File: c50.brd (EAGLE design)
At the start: 95.6 x 31.1 mm, 15 parts, among them IC1 7805TV, IC2 UA555N

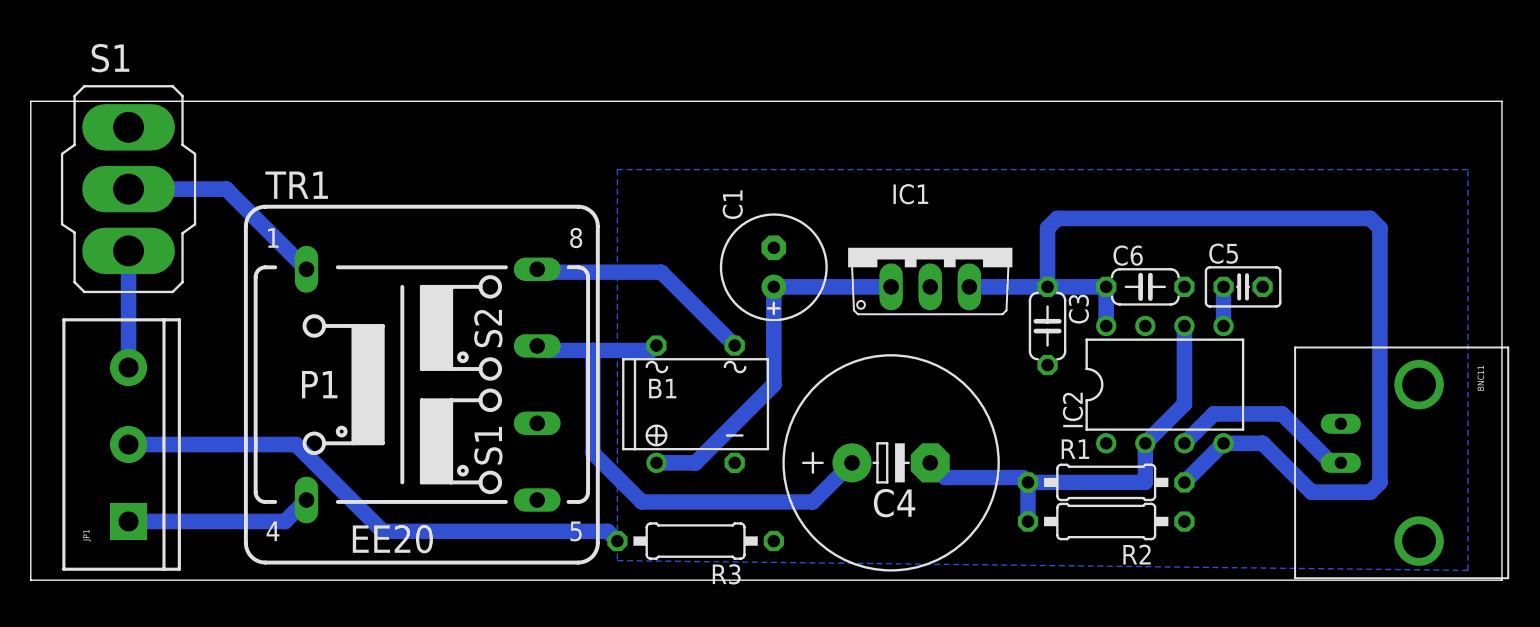
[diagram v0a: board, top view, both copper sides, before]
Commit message: Signature added.
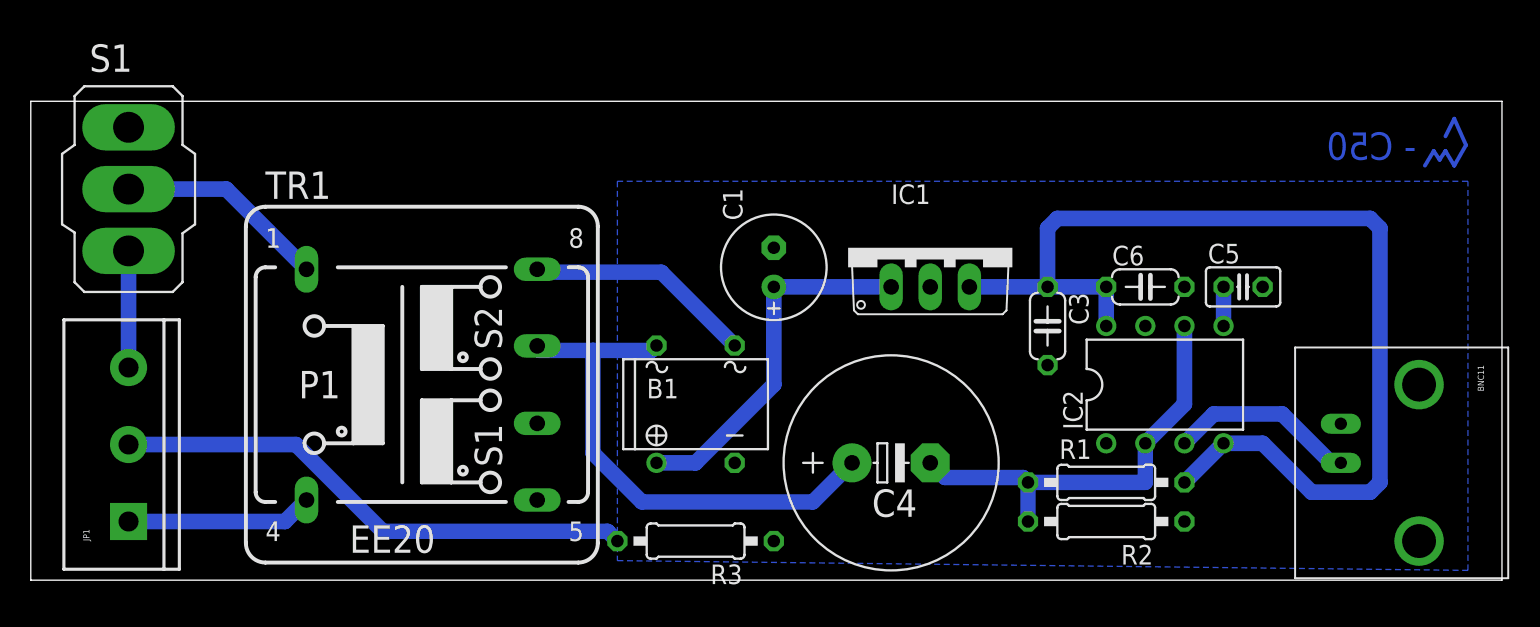
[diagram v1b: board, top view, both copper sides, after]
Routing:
- net N$11: track 0.00 -> 8.29 mm
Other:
- board text added: "- C50"
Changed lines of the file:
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@@
 <setting verticaltext="up"/>
 </settings>
-<grid distance="0.05" unitdist="inch" unit="inch" style="lines" multiple="1" display="yes" altdistance="0.0125" altunitdist="inch" altunit="inch"/>
+<grid distance="0.005" unitdist="inch" unit="inch" style="lines" multiple="1" display="yes" altdistance="0.0125" altunitdist="inch" altunit="inch"/>
 <layers>
 <layer number="1" name="Top" color="4" fill="1" visible="yes" active="yes"/>
@@
 <dimension x1="0" y1="0" x2="0" y2="31.105" x3="-4.445" y3="15.5525" textsize="1.778" layer="20"/>
 <dimension x1="0" y1="0" x2="95.555" y2="0" x3="47.7775" y3="-5.08" textsize="1.778" layer="20"/>
+<text x="90.678" y="27.305" size="1.778" layer="16" rot="MR0"> - C50</text>
 </plain>
 <attributes>
@@
 <contactref element="R3" pad="1"/>
 <polygon width="0.4064" layer="16">
-<vertex x="38.1" y="26.67"/>
+<vertex x="38.1" y="25.908"/>
 <vertex x="38.1" y="1.27"/>
 <vertex x="93.345" y="0.635"/>
-<vertex x="93.345" y="26.67"/>
+<vertex x="93.345" y="25.908"/>
 </polygon>
 </signal>
@@
 <wire x1="6.35" y1="13.81" x2="6.35" y2="21.3868" width="1.016" layer="16"/>
 </signal>
+<signal name="N$11">
+<wire x1="91.8845" y1="28.829" x2="92.456" y2="29.972" width="0.254" layer="16"/>
+<wire x1="92.456" y1="29.972" x2="93.218" y2="28.2575" width="0.254" layer="16"/>
+<wire x1="93.218" y1="28.2575" x2="92.456" y2="26.924" width="0.254" layer="16"/>
+<wire x1="92.456" y1="26.924" x2="91.8845" y2="27.8765" width="0.254" layer="16"/>
+<wire x1="91.8845" y1="27.8765" x2="91.5035" y2="27.305" width="0.254" layer="16"/>
+<wire x1="91.5035" y1="27.305" x2="91.1225" y2="27.8765" width="0.254" layer="16"/>
+<wire x1="91.1225" y1="27.8765" x2="90.551" y2="26.924" width="0.254" layer="16"/>
+</signal>
 </signals>
